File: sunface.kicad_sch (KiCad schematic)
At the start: 5 parts, among them U1 PT4115

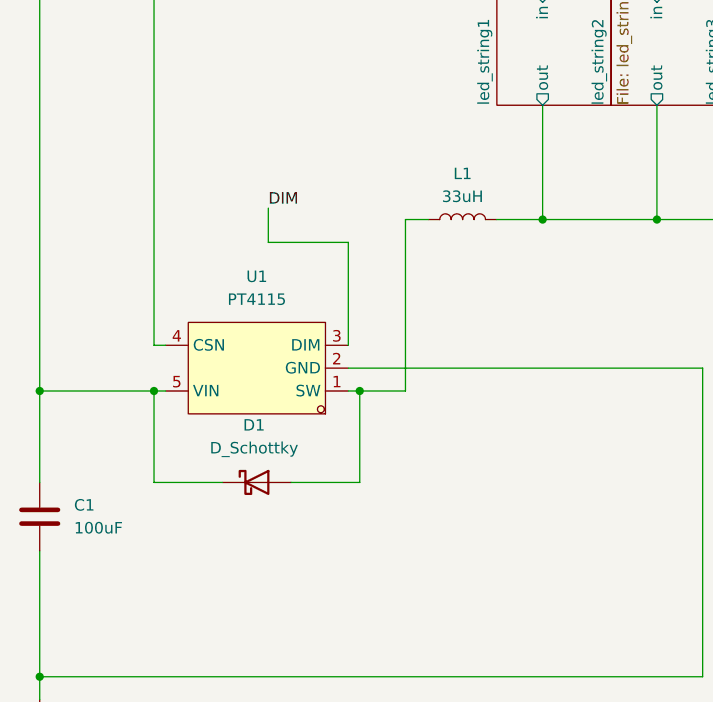
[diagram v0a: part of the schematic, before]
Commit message: finalise design for manufacture
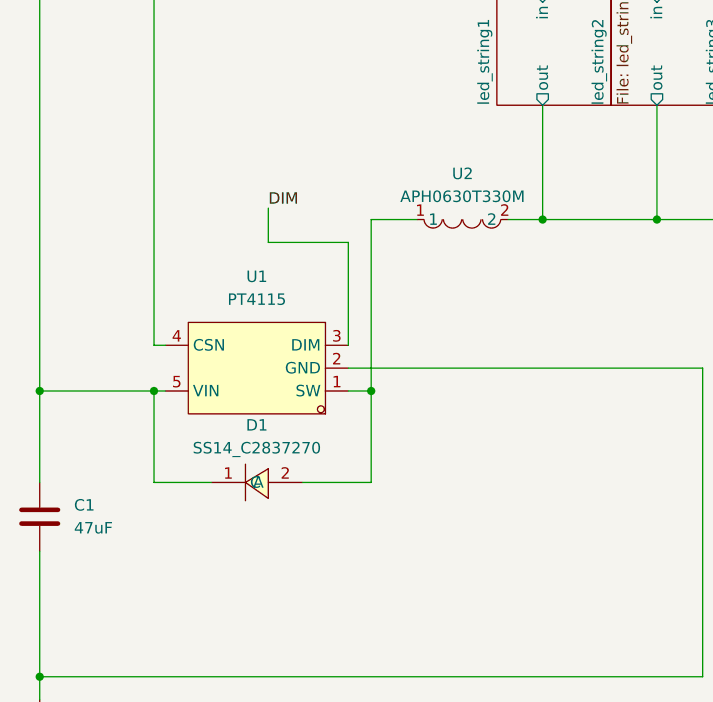
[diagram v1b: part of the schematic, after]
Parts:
- removed D1: D_Schottky, easyeda2kicad:SMA_L4.3-W2.6-LS5.0-RD, symbol Device:D_Schottky
- removed L1: 33uH, easyeda2kicad:IND-SMD_L7.1-W6.6, symbol Device:L
- added D1: SS14_C2837270, easyeda2kicad:SMA_L4.3-W2.6-LS5.0-RD, symbol easyeda2kicad:SS14_C2837270
- added U2: APH0630T330M, easyeda2kicad:IND-SMD_L7.1-W6.6, symbol easyeda2kicad:APH0630T330M
- C1: value 100uF -> 47uF
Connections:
- net 12V: now also D1.1 (C)
- net led_string1/out: now also U2.2
- net at U1.1 (SW): now also D1.2 (A), U2.1
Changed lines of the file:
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@@
-	)
-	(junction
-		(at 60.96 95.25)
-		(diameter 0)
-		(color 0 0 0 0)
 	)
 	(junction
@@
 	)
 	(junction
+		(at 62.23 95.25)
+		(diameter 0)
+		(color 0 0 0 0)
+	)
+	(junction
 		(at 106.68 38.1)
 		(diameter 0)
@@
 	(wire
 		(pts
-			(xy 53.34 105.41) (xy 60.96 105.41)
-		)
-		(stroke
-			(width 0)
-			(type default)
-		)
-	)
-	(wire
-		(pts
 			(xy 25.4 129.54) (xy 25.4 127)
 		)
@@
 	(wire
 		(pts
-			(xy 76.2 76.2) (xy 81.28 76.2)
-		)
-		(stroke
-			(width 0)
-			(type default)
-		)
-	)
-	(wire
-		(pts
 			(xy 233.68 38.1) (xy 246.38 38.1)
 		)
@@
 	(wire
 		(pts
+			(xy 62.23 76.2) (xy 67.31 76.2)
+		)
+		(stroke
+			(width 0)
+			(type default)
+		)
+	)
+	(wire
+		(pts
 			(xy 81.28 76.2) (xy 81.28 63.5)
 		)
@@
 	(wire
 		(pts
-			(xy 68.58 76.2) (xy 66.04 76.2)
-		)
-		(stroke
-			(width 0)
-			(type default)
-		)
-	)
-	(wire
-		(pts
 			(xy 93.98 38.1) (xy 106.68 38.1)
 		)
@@
 	(wire
 		(pts
-			(xy 45.72 105.41) (xy 38.1 105.41)
+			(xy 44.45 105.41) (xy 38.1 105.41)
 		)
 		(stroke
@@
 	(wire
 		(pts
-			(xy 66.04 76.2) (xy 66.04 95.25)
+			(xy 62.23 76.2) (xy 62.23 95.25)
 		)
 		(stroke
@@
 	(wire
 		(pts
-			(xy 60.96 95.25) (xy 60.96 105.41)
+			(xy 62.23 95.25) (xy 62.23 105.41)
 		)
 		(stroke
@@
 	(wire
 		(pts
-			(xy 66.04 95.25) (xy 60.96 95.25)
-		)
-		(stroke
-			(width 0)
-			(type default)
-		)
-	)
-	(wire
-		(pts
 			(xy 170.18 63.5) (xy 170.18 76.2)
 		)
@@
 	(wire
 		(pts
+			(xy 77.47 76.2) (xy 81.28 76.2)
+		)
+		(stroke
+			(width 0)
+			(type default)
+		)
+	)
+	(wire
+		(pts
 			(xy 119.38 38.1) (xy 132.08 38.1)
 		)
@@
 	(wire
 		(pts
+			(xy 54.61 105.41) (xy 62.23 105.41)
+		)
+		(stroke
+			(width 0)
+			(type default)
+		)
+	)
+	(wire
+		(pts
 			(xy 38.1 95.25) (xy 39.37 95.25)
 		)
@@
 	(wire
 		(pts
-			(xy 60.96 95.25) (xy 59.69 95.25)
+			(xy 59.69 95.25) (xy 62.23 95.25)
 		)
 		(stroke
@@
 			)
 			(justify left bottom)
+		)
+	)
+	(symbol
+		(lib_id "easyeda2kicad:APH0630T330M")
+		(at 72.39 76.2 0)
+		(unit 1)
+		(exclude_from_sim no)
+		(in_bom yes)
+		(on_board yes)
+		(dnp no)
+		(fields_autoplaced yes)
+		(property "Reference" "U2"
+			(at 72.39 71.12 0)
+			(effects
+				(font
+					(size 1.27 1.27)
+				)
+			)
+		)
+		(property "Value" "APH0630T330M"
+			(at 72.39 73.66 0)
+			(effects
+				(font
+					(size 1.27 1.27)
+				)
+			)
+		)
+		(property "Footprint" "easyeda2kicad:IND-SMD_L7.1-W6.6"
+			(at 72.39 83.82 0)
+			(effects
+				(font
+					(size 1.27 1.27)
+				)
+				(hide yes)
+			)
+		)
+		(property "Datasheet" ""
+			(at 72.39 76.2 0)
+			(effects
+				(font
+					(size 1.27 1.27)
+				)
+				(hide yes)
+			)
+		)
+		(property "Description" ""
+			(at 72.39 76.2 0)
+			(effects
+				(font
+					(size 1.27 1.27)
+				)
+				(hide yes)
+			)
+		)
+		(property "LCSC Part" "C5349704"
+			(at 72.39 86.36 0)
+			(effects
+				(font
+					(size 1.27 1.27)
+				)
+				(hide yes)
+			)
+		)
+		(pin "1"
+		)
+		(pin "2"
+		)
+		(instances
+			(project ""
+				(path "/b5279a47-4e53-4efd-ad9f-4a5619d0841f"
+					(reference "U2")
+					(unit 1)
+				)
+			)
 		)
 	)
@@
 	)
 	(symbol
-		(lib_id "Device:L")
-		(at 72.39 76.2 90)
-		(unit 1)
-		(exclude_from_sim no)
-		(in_bom yes)
-		(on_board yes)
-		(dnp no)
-		(fields_autoplaced yes)
-		(property "Reference" "L1"
-			(at 72.39 71.12 90)
-			(effects
-				(font
-					(size 1.27 1.27)
-				)
-			)
-		)
-		(property "Value" "33uH"
-			(at 72.39 73.66 90)
-			(effects
-				(font
-					(size 1.27 1.27)
-				)
-			)
-		)
-		(property "Footprint" "easyeda2kicad:IND-SMD_L7.1-W6.6"
-			(at 72.39 76.2 0)
-			(effects
-				(font
-					(size 1.27 1.27)
-				)
-				(hide yes)
-			)
-		)
-		(property "Datasheet" "~"
-			(at 72.39 76.2 0)
-			(effects
-				(font
-					(size 1.27 1.27)
-				)
-				(hide yes)
-			)
-		)
-		(property "Description" "Inductor"
-			(at 72.39 76.2 0)
-			(effects
-				(font
-					(size 1.27 1.27)
-				)
-				(hide yes)
-			)
-		)
-		(pin "1"
-		)
-		(pin "2"
-		)
-		(instances
-			(project ""
-				(path "/b5279a47-4e53-4efd-ad9f-4a5619d0841f"
-					(reference "L1")
-					(unit 1)
-				)
-			)
-		)
-	)
-	(symbol
 		(lib_id "easyeda2kicad:PT4115")
 		(at 49.53 92.71 180)
@@
 				(path "/b5279a47-4e53-4efd-ad9f-4a5619d0841f"
 					(reference "U1")
-					(unit 1)
-				)
-			)
-		)
-	)
-	(symbol
-		(lib_id "Device:D_Schottky")
-		(at 49.53 105.41 0)
-		(unit 1)
-		(exclude_from_sim no)
-		(in_bom yes)
-		(on_board yes)
-		(dnp no)
-		(fields_autoplaced yes)
-		(property "Reference" "D1"
-			(at 49.2125 99.06 0)
-			(effects
-				(font
-					(size 1.27 1.27)
-				)
-			)
-		)
-		(property "Value" "D_Schottky"
-			(at 49.2125 101.6 0)
-			(effects
-				(font
-					(size 1.27 1.27)
-				)
-			)
-		)
-		(property "Footprint" "easyeda2kicad:SMA_L4.3-W2.6-LS5.0-RD"
-			(at 49.53 105.41 0)
-			(effects
-				(font
-					(size 1.27 1.27)
-				)
-				(hide yes)
-			)
-		)
-		(property "Datasheet" "~"
-			(at 49.53 105.41 0)
-			(effects
-				(font
-					(size 1.27 1.27)
-				)
-				(hide yes)
-			)
-		)
-		(property "Description" "Schottky diode"
-			(at 49.53 105.41 0)
-			(effects
-				(font
-					(size 1.27 1.27)
-				)
-				(hide yes)
-			)
-		)
-		(pin "1"
-		)
-		(pin "2"
-		)
-		(instances
-			(project ""
-				(path "/b5279a47-4e53-4efd-ad9f-4a5619d0841f"
-					(reference "D1")
 					(unit 1)
 				)
@@
 			)
 		)
-		(property "Value" "100uF"
+		(property "Value" "47uF"
 			(at 29.21 110.4899 0)
 			(effects
@@
 					(unit 1)
 				)
+			)
+		)
+	)
+	(symbol
+		(lib_id "easyeda2kicad:SS14_C2837270")
+		(at 49.53 105.41 0)
+		(unit 1)
+		(exclude_from_sim no)
+		(in_bom yes)
+		(on_board yes)
+		(dnp no)
+		(fields_autoplaced yes)
+		(property "Reference" "D1"
+			(at 49.53 99.06 0)
+			(effects
+				(font
+					(size 1.27 1.27)
+				)
+			)
+		)
+		(property "Value" "SS14_C2837270"
+			(at 49.53 101.6 0)
+			(effects
+				(font
+					(size 1.27 1.27)
+				)
+			)
+		)
+		(property "Footprint" "easyeda2kicad:SMA_L4.3-W2.6-LS5.0-RD"
+			(at 49.53 113.03 0)
+			(effects
+				(font
+					(size 1.27 1.27)
+				)
+				(hide yes)
+			)
+		)
+		(property "Datasheet" ""
+			(at 49.53 105.41 0)
+			(effects
+				(font
+					(size 1.27 1.27)
+				)
+				(hide yes)
+			)
+		)
+		(property "Description" ""
+			(at 49.53 105.41 0)
+			(effects
+				(font
+					(size 1.27 1.27)
+				)
+				(hide yes)
+			)
+		)
+		(property "LCSC Part" "C2837270"
+			(at 49.53 115.57 0)
+			(effects
+				(font
+					(size 1.27 1.27)
+				)
+				(hide yes)
+			)
+		)
+		(pin "1"
+		)
+		(pin "2"
+		)
+		(instances
+			(project ""
+				(path "/b5279a47-4e53-4efd-ad9f-4a5619d0841f"
+					(reference "D1")
+					(unit 1)
+				)
